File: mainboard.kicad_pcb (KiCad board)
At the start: 2 copper layers, 115.3 x 64.5 mm, 13 parts

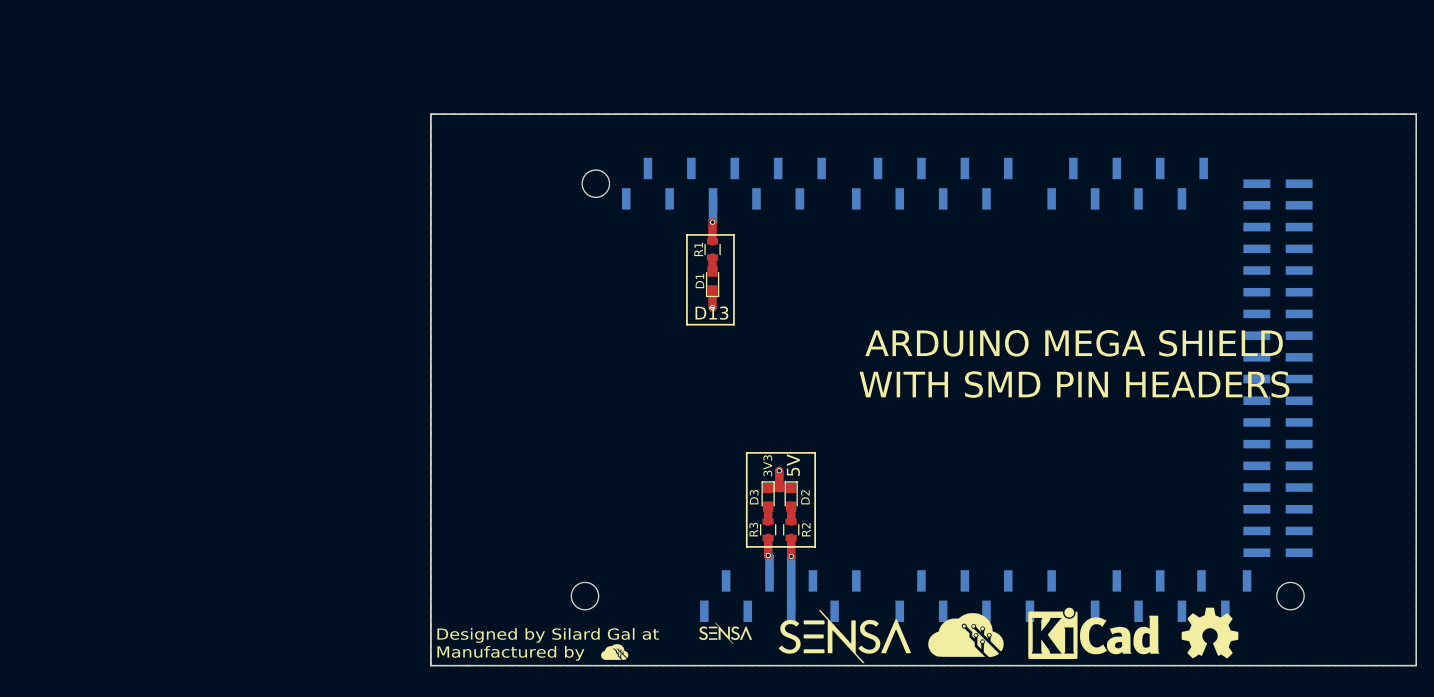
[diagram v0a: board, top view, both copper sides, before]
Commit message: Beta version
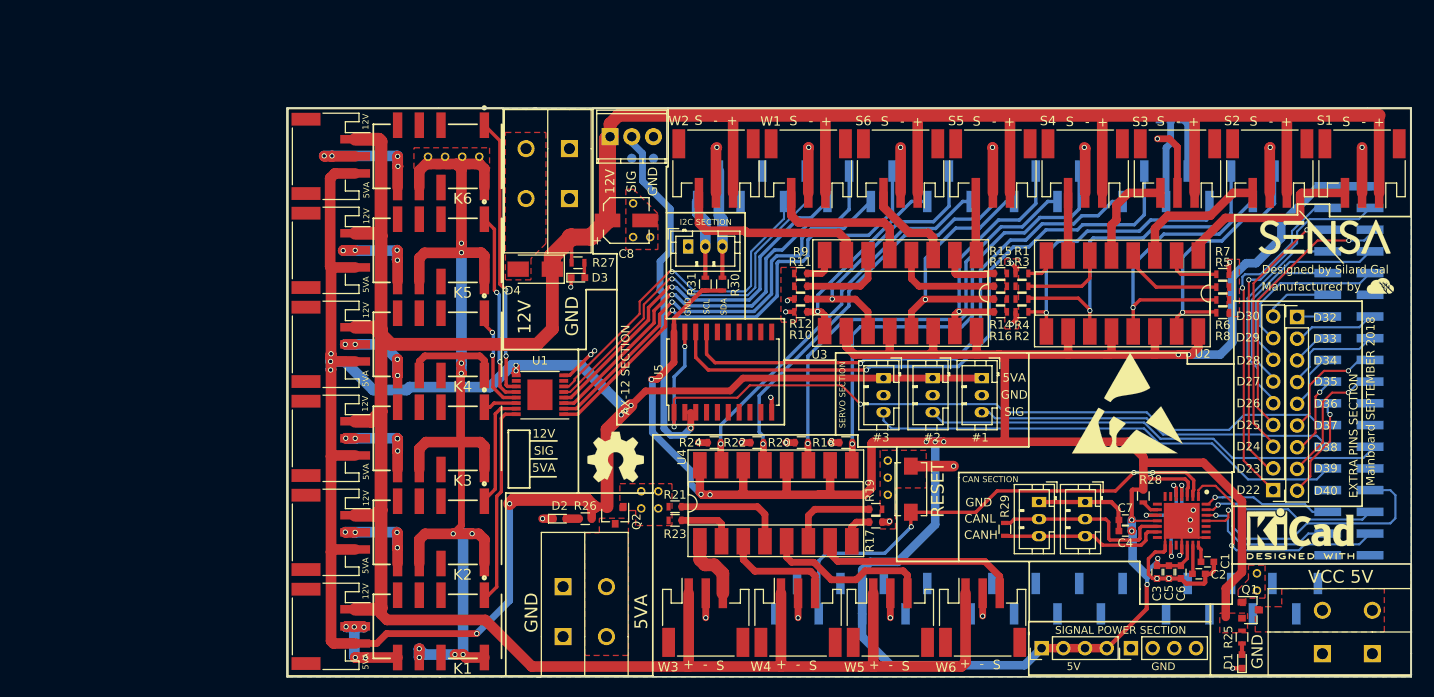
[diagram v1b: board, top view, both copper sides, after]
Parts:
- removed the G*** at (219.8, 140.8)
- removed the G*** at (191.4, 140.6)
- removed the REF*** at (234.6, 140.6)
- added C1: C, Capacitors_SMD:C_0603, F.Cu at (247.9, 132.2)
- added C2: C, Capacitors_SMD:C_0603, F.Cu at (246.9, 133.7)
- added C3: 10u, Capacitors_SMD:C_0603, F.Cu at (242.0, 133.4)
- added C4: 0.1u, Capacitors_SMD:C_0603, F.Cu at (238.3, 128.7)
- added C5: 0.1u, Capacitors_SMD:C_0603, F.Cu at (243.4, 133.4)
- added C6: 0.1u, Capacitors_SMD:C_0603, F.Cu at (244.8, 133.4)
- added C7: 0.1u, Capacitors_SMD:C_0603, F.Cu at (238.3, 127.3)
- added C8: CP, Capacitors_SMD:CP_Elec_5x5.8, F.Cu at (179.9, 92.3)
- added D4: D, Diodes_SMD:D_SMA, F.Cu at (169.2, 98.0)
- added IC1: MCP25625-E_ML, MCP25625-E_ML:QFN65P600X600X100-29N-D, F.Cu at (244.9, 127.5)
- added J1: SENS1, Connectors_JST:JST_PH_S3B-PH-SM4-TB_03x2.00mm_Angled, F.Cu at (266.0, 86.2)
- added J10: R4, Connectors_JST:JST_PH_S3B-PH-SM4-TB_03x2.00mm_Angled, F.Cu at (145.3, 106.8)
- added J11: R5, Connectors_JST:JST_PH_S3B-PH-SM4-TB_03x2.00mm_Angled, F.Cu at (145.3, 95.8)
- added J12: R6, Connectors_JST:JST_PH_S3B-PH-SM4-TB_03x2.00mm_Angled, F.Cu at (145.3, 84.8)
- added J13: SW1, Connectors_JST:JST_PH_S3B-PH-SM4-TB_03x2.00mm_Angled, F.Cu at (201.2, 86.2)
- added J14: SW2, Connectors_JST:JST_PH_S3B-PH-SM4-TB_03x2.00mm_Angled, F.Cu at (190.4, 86.2)
- added J15: SW3, Connectors_JST:JST_PH_S3B-PH-SM4-TB_03x2.00mm_Angled, F.Cu at (189.2, 138.8)
- added J16: SW4, Connectors_JST:JST_PH_S3B-PH-SM4-TB_03x2.00mm_Angled, F.Cu at (200.0, 138.8)
- added J17: SW5, Connectors_JST:JST_PH_S3B-PH-SM4-TB_03x2.00mm_Angled, F.Cu at (210.8, 138.8)
- added J18: SW6, Connectors_JST:JST_PH_S3B-PH-SM4-TB_03x2.00mm_Angled, F.Cu at (221.6, 138.8)
- added J19: Conn_01x03, Connectors_JST:JST_PH_B3B-PH-K_03x2.00mm_Straight, F.Cu at (221.5, 110.8)
- added J2: SENS2, Connectors_JST:JST_PH_S3B-PH-SM4-TB_03x2.00mm_Angled, F.Cu at (255.2, 86.2)
- added J20: Conn_01x03, Connectors_JST:JST_PH_B3B-PH-K_03x2.00mm_Straight, F.Cu at (215.8, 110.8)
- added J21: Conn_01x03, Connectors_JST:JST_PH_B3B-PH-K_03x2.00mm_Straight, F.Cu at (210.0, 110.8)
- added J22: Conn_01x03, Connectors_JST:JST_PH_B3B-PH-K_03x2.00mm_Straight, F.Cu at (187.2, 95.3)
- added J23: Screw_Terminal_01x02, Custom Connector:ZFKDS, F.Cu at (267.2, 143.0)
- added J24: Screw_Terminal_01x02, Custom Connector:ZFKDS, F.Cu at (172.5, 141.0)
- added J25: Screw_Terminal_01x02, Custom Connector:ZFKDS, F.Cu at (173.2, 83.9)
- added J26: Conn_01x03, Connectors_JST:JST_PH_B3B-PH-K_03x2.00mm_Straight, F.Cu at (233.6, 125.2)
- added J27: Conn_01x03, Connectors_JST:JST_PH_B3B-PH-K_03x2.00mm_Straight, F.Cu at (228.2, 125.2)
- added J28: Conn_01x04, Pin_Headers:Pin_Header_Straight_1x04_Pitch2.54mm, F.Cu at (228.5, 142.3)
- added J29: Conn_01x03, Connectors:GS3, B.Cu at (243.6, 80.3)
- added J3: SENS3, Connectors_JST:JST_PH_S3B-PH-SM4-TB_03x2.00mm_Angled, F.Cu at (244.4, 86.2)
- added J30: Screw_Terminal_01x03, TerminalBlocks_Phoenix:TerminalBlock_Phoenix_MPT-2.54mm_3pol, F.Cu at (178.0, 82.5)
- added J31: Conn_01x04, Pin_Headers:Pin_Header_Straight_1x04_Pitch2.54mm, F.Cu at (238.9, 142.3)
- added J32: Conn_01x10, Pin_Headers:Pin_Header_Straight_1x09_Pitch2.54mm, F.Cu at (255.6, 123.8)
- added J33: Conn_01x10, Pin_Headers:Pin_Header_Straight_1x09_Pitch2.54mm, F.Cu at (258.4, 103.6)
- added J4: SENS4, Connectors_JST:JST_PH_S3B-PH-SM4-TB_03x2.00mm_Angled, F.Cu at (233.6, 86.2)
- added J5: SENS5, Connectors_JST:JST_PH_S3B-PH-SM4-TB_03x2.00mm_Angled, F.Cu at (222.8, 86.2)
- added J6: SENS6, Connectors_JST:JST_PH_S3B-PH-SM4-TB_03x2.00mm_Angled, F.Cu at (212.0, 86.2)
- added J7: R1, Connectors_JST:JST_PH_S3B-PH-SM4-TB_03x2.00mm_Angled, F.Cu at (145.3, 139.8)
- added J8: R2, Connectors_JST:JST_PH_S3B-PH-SM4-TB_03x2.00mm_Angled, F.Cu at (145.3, 128.8)
- added J9: R3, Connectors_JST:JST_PH_S3B-PH-SM4-TB_03x2.00mm_Angled, F.Cu at (145.3, 117.8)
- added K1: EE2-5NU, EE2-5NU, F.Cu at (165.3, 139.8)
- added K2: EE2-5NU, EE2-5NU, F.Cu at (165.3, 128.8)
- added K3: EE2-5NU, EE2-5NU, F.Cu at (165.3, 117.8)
- added K4: EE2-5NU, EE2-5NU, F.Cu at (165.3, 106.8)
- added K5: EE2-5NU, EE2-5NU, F.Cu at (165.3, 95.8)
- added K6: EE2-5NU, EE2-5NU, F.Cu at (165.3, 84.8)
- added Q1: DMP2100U, TO_SOT_Packages_SMD:SOT-23, F.Cu at (252.9, 137.9)
- added Q2: DMP2100U, TO_SOT_Packages_SMD:SOT-23, F.Cu at (178.6, 126.8)
- added R10: 4k7, Resistors_SMD:R_0603, F.Cu at (200.3, 103.0)
- added R11: 330, Resistors_SMD:R_0603, F.Cu at (200.3, 100.0)
- added R12: 4k7, Resistors_SMD:R_0603, F.Cu at (200.3, 101.5)
- added R13: 330, Resistors_SMD:R_0603, F.Cu at (223.7, 100.0)
- added R14: 4k7, Resistors_SMD:R_0603, F.Cu at (223.7, 101.5)
- added R15: 330, Resistors_SMD:R_0603, F.Cu at (223.7, 98.5)
- added R16: 4k7, Resistors_SMD:R_0603, F.Cu at (223.7, 103.0)
- added R17: 330, Resistors_SMD:R_0603, F.Cu at (209.1, 127.6)
- added R18: 4k7, Resistors_SMD:R_0603, F.Cu at (205.6, 118.3)
- added R19: 330, Resistors_SMD:R_0603, F.Cu at (209.1, 126.1)
- added R20: 4k7, Resistors_SMD:R_0603, F.Cu at (200.4, 118.3)
- added R21: 330, Resistors_SMD:R_0603, F.Cu at (185.6, 125.8)
- added R22: 4k7, Resistors_SMD:R_0603, F.Cu at (195.2, 118.3)
- added R23: 330, Resistors_SMD:R_0603, F.Cu at (185.6, 127.4)
- added R24: 4k7, Resistors_SMD:R_0603, F.Cu at (190.2, 118.3)
- added R25: 330, Resistors_SMD:R_0603, F.Cu at (251.9, 141.1)
- added R26: 330, Resistors_SMD:R_0603, F.Cu at (175.1, 127.2)
- added R27: 1K, Resistors_SMD:R_0603, F.Cu at (174.2, 97.2)
- added R28: 10k, Resistors_SMD:R_0603, F.Cu at (240.4, 124.5)
- added R29: 120, Resistors_SMD:R_0603, F.Cu at (224.2, 128.4)
- added R30: 4k7, Resistors_SMD:R_0603, F.Cu at (191.2, 99.8)
- added R31: 4k7, Resistors_SMD:R_0603, F.Cu at (189.2, 99.8)
- added R4: 4k7, Resistors_SMD:R_0603, F.Cu at (226.2, 101.5)
- added R5: 330, Resistors_SMD:R_0603, F.Cu at (249.7, 100.1)
- added R6: 4k7, Resistors_SMD:R_0603, F.Cu at (249.7, 101.6)
- added R7: 330, Resistors_SMD:R_0603, F.Cu at (249.7, 98.6)
- added R8: 4k7, Resistors_SMD:R_0603, F.Cu at (249.7, 103.1)
- added R9: 330, Resistors_SMD:R_0603, F.Cu at (200.3, 98.5)
- added REF**: SolderWirePad_single_1mmDrill, Wire_Pads:SolderWirePad_single_1mmDrill, F.Cu at (182.7, 94.2)
- added REF**: SolderWirePad_single_1mmDrill, Wire_Pads:SolderWirePad_single_1mmDrill, F.Cu at (253.7, 135.6)
- added REF**: SolderWirePad_single_1mmDrill, Wire_Pads:SolderWirePad_single_1mmDrill, F.Cu at (183.7, 126.0)
- added REF**: SolderWirePad_single_1mmDrill, Wire_Pads:SolderWirePad_single_1mmDrill, F.Cu at (181.7, 126.0)
- added REF**: SolderWirePad_single_1mmDrill, Wire_Pads:SolderWirePad_single_1mmDrill, F.Cu at (210.5, 120.4)
- added REF**: SolderWirePad_single_1mmDrill, Wire_Pads:SolderWirePad_single_1mmDrill, F.Cu at (253.7, 133.6)
- added REF**: SolderWirePad_single_1mmDrill, Wire_Pads:SolderWirePad_single_1mmDrill, F.Cu at (183.7, 124.0)
- added REF**: SolderWirePad_single_1mmDrill, Wire_Pads:SolderWirePad_single_1mmDrill, F.Cu at (181.7, 124.0)
- added REF**: SolderWirePad_single_1mmDrill, Wire_Pads:SolderWirePad_single_1mmDrill, F.Cu at (180.7, 94.2)
- added REF**: SolderWirePad_single_1mmDrill, Wire_Pads:SolderWirePad_single_1mmDrill, F.Cu at (180.7, 90.3)
- added REF**: SolderWirePad_single_1mmDrill, Wire_Pads:SolderWirePad_single_1mmDrill, F.Cu at (162.7, 84.8)
- added REF**: SolderWirePad_single_1mmDrill, Wire_Pads:SolderWirePad_single_1mmDrill, F.Cu at (160.7, 84.8)
- added REF**: SolderWirePad_single_1mmDrill, Wire_Pads:SolderWirePad_single_1mmDrill, F.Cu at (158.7, 84.8)
- added REF**: SolderWirePad_single_1mmDrill, Wire_Pads:SolderWirePad_single_1mmDrill, F.Cu at (156.7, 84.8)
- added REF**: SolderWirePad_single_1mmDrill, Wire_Pads:SolderWirePad_single_1mmDrill, F.Cu at (210.5, 124.4)
- added REF**: SolderWirePad_single_1mmDrill, Wire_Pads:SolderWirePad_single_1mmDrill, F.Cu at (210.5, 122.4)
- added REF***: ESD-Logo_13.2x12mm_SilkScreen, Symbols:ESD-Logo_13.2x12mm_SilkScreen, F.Cu at (238.6, 113.7)
- added REF***: KiCad-Logo2_6mm_SilkScreen, Symbols:KiCad-Logo2_6mm_SilkScreen, F.Cu at (258.8, 128.9)
- added SW1: SW_Push, Buttons_Switches_SMD:SW_SPST_EVQPE1, F.Cu at (213.2, 123.8)
- added U1: ULN2003A, Housings_SSOP:TSSOP-16-1EP_4.4x5mm_Pitch0.65mm, F.Cu at (169.8, 112.7)
- added U2: LTV-847, Housings_DIP:DIP-16_W8.89mm_SMDSocket_LongPads, F.Cu at (237.9, 100.8)
- added U3: LTV-847, Housings_DIP:DIP-16_W8.89mm_SMDSocket_LongPads, F.Cu at (212.0, 100.8)
- added U4: LTV-847, Housings_DIP:DIP-16_W8.89mm_SMDSocket_LongPads, F.Cu at (197.4, 125.4)
- added U5: 74LS241, Housings_SOIC:SOIC-20W_7.5x12.8mm_Pitch1.27mm, F.Cu at (191.2, 110.0)
- D1, D2, D3: footprint LEDs:LED_0805 -> LEDs:LED_0603
- R1, R3: value R -> 330; footprint Resistors_SMD:R_0805 -> Resistors_SMD:R_0603
- R2: value R -> 4k7; footprint Resistors_SMD:R_0805 -> Resistors_SMD:R_0603
- moved G*** 99.3 mm to (268.2, 100.0)
- moved D1 76.3 mm to (251.9, 143.9)
- moved G*** 73.1 mm to (261.4, 94.2)
- moved REF*** 72.5 mm to (178.7, 120.0)
- moved R3 41.2 mm to (226.2, 100.0), turned to 0 degrees
- moved R2 37.1 mm to (226.2, 103.0), turned to 180 degrees
- moved R1 36.3 mm to (226.2, 98.5), turned to 0 degrees
- moved D3 34.0 mm to (174.2, 99.0), turned to 0 degrees
- moved D2 27.2 mm to (172.1, 127.2), turned to 0 degrees
- moved XA1 8.31 mm to (169.4, 139.1)
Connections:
- R1 pad 1: D13 -> GND
- R1 pad 2: Net-(D1-Pad2) -> Net-(R1-Pad2)
- R2 pad 1: +5V -> SO_4
- R2 pad 2: Net-(D2-Pad2) -> GND
- R3 pad 1: +3V3 -> GND
- R3 pad 2: Net-(D3-Pad2) -> Net-(R3-Pad2)
- XA1 pad 3V3: +3V3 -> (no net)
- XA1 pad D0: (no net) -> SWO_6
- XA1 pad D1: (no net) -> SWO_5
- XA1 pad D10: (no net) -> R3_CONT
- XA1 pad D11: (no net) -> R4_CONT
- XA1 pad D12: (no net) -> R5_CONT
- XA1 pad D13: D13 -> R6_CONT
- XA1 pad D14: (no net) -> AX_TX
- XA1 pad D15: (no net) -> AX_RX
- XA1 pad D16: (no net) -> DBG_TX
- XA1 pad D17: (no net) -> DBG_RX
- XA1 pad D18: (no net) -> SO_4
- XA1 pad D19: (no net) -> SO_3
- XA1 pad D2: (no net) -> SO_5
- XA1 pad D20: (no net) -> SO_2
- XA1 pad D21: (no net) -> SO_1
- XA1 pad D22: (no net) -> Net-(J32-Pad1)
- XA1 pad D23: (no net) -> Net-(J32-Pad2)
- XA1 pad D24: (no net) -> Net-(J32-Pad3)
- XA1 pad D25: (no net) -> Net-(J32-Pad4)
- XA1 pad D26: (no net) -> Net-(J32-Pad5)
- XA1 pad D27: (no net) -> Net-(J32-Pad6)
- XA1 pad D28: (no net) -> Net-(J32-Pad7)
- XA1 pad D29: (no net) -> Net-(J32-Pad8)
- XA1 pad D3: (no net) -> SO_6
- XA1 pad D30: (no net) -> Net-(J32-Pad9)
- XA1 pad D32: (no net) -> Net-(J33-Pad1)
- XA1 pad D33: (no net) -> Net-(J33-Pad2)
- XA1 pad D34: (no net) -> Net-(J33-Pad3)
- XA1 pad D35: (no net) -> Net-(J33-Pad4)
- XA1 pad D36: (no net) -> Net-(J33-Pad5)
- XA1 pad D37: (no net) -> Net-(J33-Pad6)
- XA1 pad D38: (no net) -> Net-(J33-Pad7)
- XA1 pad D39: (no net) -> Net-(J33-Pad8)
- XA1 pad D4: (no net) -> SWO_4
- XA1 pad D40: (no net) -> Net-(J33-Pad9)
- XA1 pad D42: (no net) -> AX_CONTROL
- XA1 pad D44: (no net) -> PWM1
- XA1 pad D45: (no net) -> PWM2
- XA1 pad D46: (no net) -> PWM3
- XA1 pad D49: (no net) -> CAN_INT
- XA1 pad D5: (no net) -> SWO_3
- XA1 pad D50: (no net) -> CAN_MISO
- XA1 pad D51: (no net) -> CAN_MOSI
- XA1 pad D52: (no net) -> CAN_SCK
- XA1 pad D53: (no net) -> CAN_CS
- XA1 pad D6: (no net) -> SWO_1
- XA1 pad D7: (no net) -> SWO_2
- XA1 pad D8: (no net) -> R1_CONT
- XA1 pad D9: (no net) -> R2_CONT
- XA1 pad GND1: (no net) -> GND
- XA1 pad GND2: (no net) -> GND
- XA1 pad GND3: (no net) -> GND
- XA1 pad GND5: (no net) -> GND
- XA1 pad GND6: (no net) -> GND
- XA1 pad RST1: (no net) -> RST
- XA1 pad SCL: (no net) -> SCL
- XA1 pad SDA: (no net) -> SDA
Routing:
- net +12V: track 0.00 -> 404.7 mm
- net +5V: track 8.59 -> 353.5 mm, vias 1 -> 12
- net +5VA: track 0.00 -> 269.2 mm, vias 0 -> 10
- net GND: track 6.70 -> 274.9 mm, vias 2 -> 45
- net AX_CONTROL: track 0.00 -> 95.4 mm, vias 0 -> 3
- net AX_RX: track 0.00 -> 73.1 mm, vias 0 -> 1
- net AX_TX: track 0.00 -> 64.0 mm, vias 0 -> 1
- net RST: track 0.00 -> 57.7 mm, vias 0 -> 3
- net R1_CONT: track 0.00 -> 57.7 mm, vias 0 -> 1
- net PWM3: track 0.00 -> 56.3 mm
- net SWO_6: track 0.00 -> 56.2 mm, vias 0 -> 1
- net PWM2: track 0.00 -> 55.7 mm
- net SWO_5: track 0.00 -> 53.3 mm, vias 0 -> 1
- net R3_CONT: track 0.00 -> 51.5 mm, vias 0 -> 1
- net R2_CONT: track 0.00 -> 50.9 mm, vias 0 -> 1
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- added copper zone on F.Cu, net +5V
- added copper zone on F.Cu, net GND
- added copper zone on F.Cu, net Net-(D4-Pad2)
- added copper zone on F.Cu, net Net-(J23-Pad2)
- added copper zone on F.Cu, net Net-(J24-Pad2)
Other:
- board size 115.3 x 64.5 mm -> 131.6 x 66.5 mm
- board text added: "#1"
- board text added: "#2"
- board text added: "#3"
- board text added: "+"
- board text added: "-"
- board text added: "12V"
- board text added: "5VA"
- board text added: "AX-12 SECTION"
- board text added: "CAN SECTION"
- board text added: "CANH"
- board text added: "CANL"
- board text added: "D22"
- board text added: "D23"
- board text added: "D24"
- board text added: "D25"
- board text added: "D26"
- board text added: "D27"
- board text added: "D28"
- board text added: "D29"
- board text added: "D30"
- board text added: "D32"
- board text added: "D33"
- board text added: "D34"
- board text added: "D35"
- board text added: "D36"
- board text added: "D37"
- board text added: "D38"
- board text added: "D39"
- board text added: "D40"
- board text added: "Designed by Silard Gal"
- board text added: "EXTRA PINS SECTION"
- board text added: "GND"
- board text added: "I2C SECTION"
- board text added: "Mainboard SEPTEMBER 2018"
- board text added: "Manufactured by"
- board text added: "RESET"
- board text added: "S"
- board text added: "S1"
- board text added: "S2"
- board text added: "S3"
- board text added: "S4"
- board text added: "S5"
- board text added: "S6"
- board text added: "SCL"
- board text added: "SDA"
- board text added: "SERVO SECTION"
- board text added: "SIG"
- board text added: "SIGNAL POWER SECTION"
- board text added: "VCC 5V"
- board text added: "W1"
- board text added: "W2"
- board text added: "W3"
- board text added: "W4"
- board text added: "W5"
- board text added: "W6"
- board text removed: "3V3"
- board text removed: "ARDUINO MEGA SHIELD WITH SMD PIN HEADERS"
- board text removed: "D13"
- board text removed: "Designed by Silard Gal at Manufactured by"

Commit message: Finished version 1.0
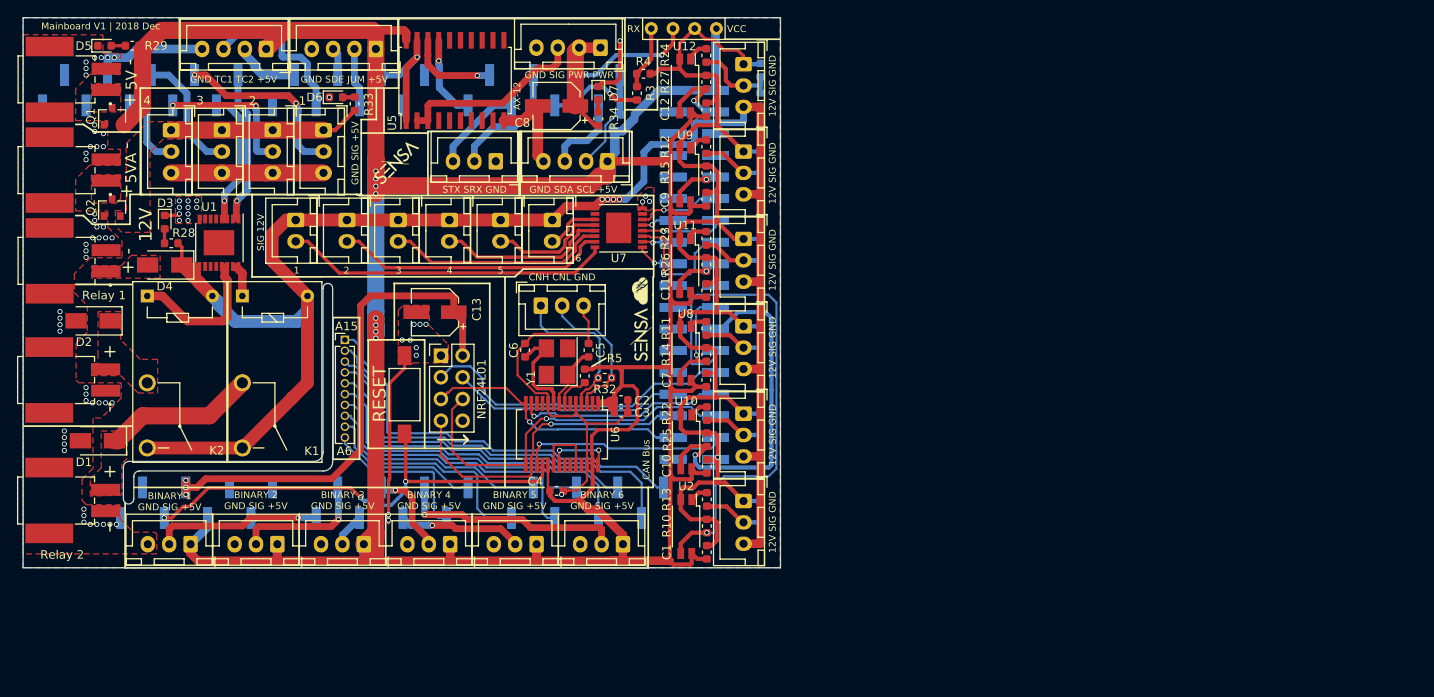
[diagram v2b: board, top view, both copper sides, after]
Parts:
- removed IC1: MCP25625-E_ML, MCP25625-E_ML:QFN65P600X600X100-29N-D
- removed J16: SW4, Connectors_JST:JST_PH_S3B-PH-SM4-TB_03x2.00mm_Angled
- removed J29: Conn_01x03, Connectors:GS3
- removed K3, K4, K5, K6: EE2-5NU, EE2-5NU
- removed REF** (x16): SolderWirePad_single_1mmDrill, Wire_Pads:SolderWirePad_single_1mmDrill
- removed REF***: ESD-Logo_13.2x12mm_SilkScreen, Symbols:ESD-Logo_13.2x12mm_SilkScreen
- removed REF***: KiCad-Logo2_6mm_SilkScreen, Symbols:KiCad-Logo2_6mm_SilkScreen
- removed REF***: OSHW-Symbol_6.7x6mm_SilkScreen, Symbols:OSHW-Symbol_6.7x6mm_SilkScreen
- removed SW1: SW_Push, Buttons_Switches_SMD:SW_SPST_EVQPE1
- removed the XA1 at (169.4, 139.1)
- added C10: 100n, Capacitor_SMD:C_0603_1608Metric, F.Cu at (189.3, 121.1)
- added C11: 100n, Capacitor_SMD:C_0603_1608Metric, F.Cu at (189.3, 100.5)
- added C12: 100n, Capacitor_SMD:C_0603_1608Metric, F.Cu at (189.3, 79.3)
- added C13: CP, Capacitor_SMD:CP_Elec_5x5.8, F.Cu at (157.5, 103.0)
- added C9: 100n, Capacitor_SMD:C_0603_1608Metric, F.Cu at (189.3, 89.8)
- added D5: LED, LED_SMD:LED_0603_1608Metric, F.Cu at (118.8, 71.9)
- added D6: LED, LED_SMD:LED_0603_1608Metric, F.Cu at (145.9, 77.9)
- added D7: LED, LED_SMD:LED_0603_1608Metric, F.Cu at (176.6, 77.4)
- added G***: LOGO, logos:SENSA_6x3, F.Cu at (152.9, 85.5)
- added G***: LOGO, logos:SENSA_6x3, F.Cu at (181.6, 105.8)
- added G***: LOGO, logos:AISLER_9x5, B.Cu at (173.0, 119.0)
- added J34: SERVO4, Connector_JST:JST_XH_B03B-XH-A_1x03_P2.50mm_Vertical, F.Cu at (126.6, 81.7)
- added J35: RELAY2, PHOENIX_1702473, F.Cu at (113.2, 111.0)
- added J36: RELAY1, PHOENIX_1702473, F.Cu at (113.2, 125.1)
- added R32: 120, Resistor_SMD:R_0603_1608Metric, F.Cu at (177.4, 110.7)
- added R33: 1K, Resistor_SMD:R_0603_1608Metric, F.Cu at (148.1, 78.7)
- added R34: 1K, Resistor_SMD:R_0603_1608Metric, F.Cu at (176.6, 80.4)
- added RESET1: SW_Push, Button_Switch_SMD:SW_SPST_FSMSM, F.Cu at (154.0, 112.7)
- added U10: PC817, Package_SO:SOP-4_4.4x2.8mm_P1.27mm, F.Cu at (186.9, 118.2)
- added U11: PC817, Package_SO:SOP-4_4.4x2.8mm_P1.27mm, F.Cu at (186.8, 97.6)
- added U12: PC817, Package_SO:SOP-4_4.4x2.8mm_P1.27mm, F.Cu at (186.8, 76.6)
- added U6: MCP25625-x-SS, Package_SO:SSOP-28_5.3x10.2mm_P0.65mm, F.Cu at (172.4, 117.3)
- added U7: ULN2003A, Package_SO:TSSOP-16-1EP_4.4x5mm_P0.65mm, F.Cu at (179.0, 93.2)
- added U8: PC817, Package_SO:SOP-4_4.4x2.8mm_P1.27mm, F.Cu at (186.9, 107.9)
- added U9: PC817, Package_SO:SOP-4_4.4x2.8mm_P1.27mm, F.Cu at (186.8, 87.0)
- added XA1 (x2): Arduino_Mega2560_Shield, Arduino:Arduino_Mega2560_Shield, F.Cu at (92.8, 127.9)
- added Y1: Crystal_GND24, Crystal:Crystal_SMD_SeikoEpson_FA238V-4Pin_3.2x2.5mm_HandSoldering, F.Cu at (171.8, 108.8)
- C1: value C -> 100n; footprint Capacitors_SMD:C_0603 -> Capacitor_SMD:C_0603_1608Metric
- C2: value C -> 10u; footprint Capacitors_SMD:C_0603 -> Capacitor_SMD:C_0603_1608Metric
- C3: value 10u -> 100n; footprint Capacitors_SMD:C_0603 -> Capacitor_SMD:C_0603_1608Metric
- C4: value 0.1u -> 10u; footprint Capacitors_SMD:C_0603 -> Capacitor_SMD:C_0603_1608Metric
- C5, C6: value 0.1u -> 20p; footprint Capacitors_SMD:C_0603 -> Capacitor_SMD:C_0603_1608Metric
- C7: value 0.1u -> 100n; footprint Capacitors_SMD:C_0603 -> Capacitor_SMD:C_0603_1608Metric
- C8: footprint Capacitors_SMD:CP_Elec_5x5.8 -> Capacitor_SMD:CP_Elec_5x5.8
- D1, D2: value LED -> D; footprint LEDs:LED_0603 -> Diode_SMD:D_SMA
- D3: footprint LEDs:LED_0603 -> LED_SMD:LED_0603_1608Metric
- D4: footprint Diodes_SMD:D_SMA -> Diode_SMD:D_SMA
- G***: moved to B.Cu
- J1: value SENS1 -> Conn_01x10; footprint Connectors_JST:JST_PH_S3B-PH-SM4-TB_03x2.00mm_Angled -> Connector_PinHeader_1.27mm:PinHeader_1x10_P1.27mm_Vertical
- J10: value R4 -> jump_side; footprint Connectors_JST:JST_PH_S3B-PH-SM4-TB_03x2.00mm_Angled -> Connector_JST:JST_XH_B04B-XH-A_1x04_P2.50mm_Vertical
- J11: value R5 -> Senzor1; footprint Connectors_JST:JST_PH_S3B-PH-SM4-TB_03x2.00mm_Angled -> Connector_JST:JST_XH_B03B-XH-A_1x03_P2.50mm_Vertical
- J12: value R6 -> tactics_sw; footprint Connectors_JST:JST_PH_S3B-PH-SM4-TB_03x2.00mm_Angled -> Connector_JST:JST_XH_B04B-XH-A_1x04_P2.50mm_Vertical
- J13: value SW1 -> i2c_con; footprint Connectors_JST:JST_PH_S3B-PH-SM4-TB_03x2.00mm_Angled -> Connector_JST:JST_XH_B04B-XH-A_1x04_P2.50mm_Vertical
- J14: value SW2 -> ser_con; footprint Connectors_JST:JST_PH_S3B-PH-SM4-TB_03x2.00mm_Angled -> Connector_JST:JST_XH_B03B-XH-A_1x03_P2.50mm_Vertical
- J15: value SW3 -> CAN; footprint Connectors_JST:JST_PH_S3B-PH-SM4-TB_03x2.00mm_Angled -> Connector_JST:JST_XH_B03B-XH-A_1x03_P2.50mm_Vertical
- J17: value SW5 -> Senzor3; footprint Connectors_JST:JST_PH_S3B-PH-SM4-TB_03x2.00mm_Angled -> Connector_JST:JST_XH_B03B-XH-A_1x03_P2.50mm_Vertical
- J18: value SW6 -> Senzor5; footprint Connectors_JST:JST_PH_S3B-PH-SM4-TB_03x2.00mm_Angled -> Connector_JST:JST_XH_B03B-XH-A_1x03_P2.50mm_Vertical
- J19: value Conn_01x03 -> SERVO1; footprint Connectors_JST:JST_PH_B3B-PH-K_03x2.00mm_Straight -> Connector_JST:JST_XH_B03B-XH-A_1x03_P2.50mm_Vertical
- J2: value SENS2 -> AX; footprint Connectors_JST:JST_PH_S3B-PH-SM4-TB_03x2.00mm_Angled -> Connector_JST:JST_XH_B04B-XH-A_1x04_P2.50mm_Vertical
- J20: value Conn_01x03 -> SERVO2; footprint Connectors_JST:JST_PH_B3B-PH-K_03x2.00mm_Straight -> Connector_JST:JST_XH_B03B-XH-A_1x03_P2.50mm_Vertical
- J21: value Conn_01x03 -> S2; footprint Connectors_JST:JST_PH_B3B-PH-K_03x2.00mm_Straight -> Connector_JST:JST_XH_B02B-XH-A_1x02_P2.50mm_Vertical
- J22: value Conn_01x03 -> S3; footprint Connectors_JST:JST_PH_B3B-PH-K_03x2.00mm_Straight -> Connector_JST:JST_XH_B02B-XH-A_1x02_P2.50mm_Vertical
- J23: value Screw_Terminal_01x02 -> 12V_IN; footprint Custom Connector:ZFKDS -> PHOENIX_1702473
- J24: value Screw_Terminal_01x02 -> 5V_IN; footprint Custom Connector:ZFKDS -> PHOENIX_1702473
- J25: value Screw_Terminal_01x02 -> 5VA_IN; footprint Custom Connector:ZFKDS -> PHOENIX_1702473
- J26: value Conn_01x03 -> S4; footprint Connectors_JST:JST_PH_B3B-PH-K_03x2.00mm_Straight -> Connector_JST:JST_XH_B02B-XH-A_1x02_P2.50mm_Vertical
- J27: value Conn_01x03 -> S5; footprint Connectors_JST:JST_PH_B3B-PH-K_03x2.00mm_Straight -> Connector_JST:JST_XH_B02B-XH-A_1x02_P2.50mm_Vertical
- J28: value Conn_01x04 -> S6; footprint Pin_Headers:Pin_Header_Straight_1x04_Pitch2.54mm -> Connector_JST:JST_XH_B02B-XH-A_1x02_P2.50mm_Vertical
- J3: value SENS3 -> bin_sens1; footprint Connectors_JST:JST_PH_S3B-PH-SM4-TB_03x2.00mm_Angled -> Connector_JST:JST_XH_B03B-XH-A_1x03_P2.50mm_Vertical
- J30: value Screw_Terminal_01x03 -> Senzor2; footprint TerminalBlocks_Phoenix:TerminalBlock_Phoenix_MPT-2.54mm_3pol -> Connector_JST:JST_XH_B03B-XH-A_1x03_P2.50mm_Vertical
- J31: value Conn_01x04 -> Senzor4; footprint Pin_Headers:Pin_Header_Straight_1x04_Pitch2.54mm -> Connector_JST:JST_XH_B03B-XH-A_1x03_P2.50mm_Vertical
- J32: value Conn_01x10 -> Senzor6; footprint Pin_Headers:Pin_Header_Straight_1x09_Pitch2.54mm -> Connector_JST:JST_XH_B03B-XH-A_1x03_P2.50mm_Vertical
- J33: value Conn_01x10 -> SERVO3; footprint Pin_Headers:Pin_Header_Straight_1x09_Pitch2.54mm -> Connector_JST:JST_XH_B03B-XH-A_1x03_P2.50mm_Vertical
- J4: value SENS4 -> bin_sens4; footprint Connectors_JST:JST_PH_S3B-PH-SM4-TB_03x2.00mm_Angled -> Connector_JST:JST_XH_B03B-XH-A_1x03_P2.50mm_Vertical
- J5: value SENS5 -> S1; footprint Connectors_JST:JST_PH_S3B-PH-SM4-TB_03x2.00mm_Angled -> Connector_JST:JST_XH_B02B-XH-A_1x02_P2.50mm_Vertical
- J6: value SENS6 -> bin_sens2; footprint Connectors_JST:JST_PH_S3B-PH-SM4-TB_03x2.00mm_Angled -> Connector_JST:JST_XH_B03B-XH-A_1x03_P2.50mm_Vertical
- J7: value R1 -> bin_sens5; footprint Connectors_JST:JST_PH_S3B-PH-SM4-TB_03x2.00mm_Angled -> Connector_JST:JST_XH_B03B-XH-A_1x03_P2.50mm_Vertical
- J8: value R2 -> bin_sens3; footprint Connectors_JST:JST_PH_S3B-PH-SM4-TB_03x2.00mm_Angled -> Connector_JST:JST_XH_B03B-XH-A_1x03_P2.50mm_Vertical
- J9: value R3 -> bin_sens6; footprint Connectors_JST:JST_PH_S3B-PH-SM4-TB_03x2.00mm_Angled -> Connector_JST:JST_XH_B03B-XH-A_1x03_P2.50mm_Vertical
- K1, K2: value EE2-5NU -> G5Q-1A; footprint EE2-5NU -> Relay_THT:Relay_SPST_Omron-G5Q-1A
- Q1, Q2: footprint TO_SOT_Packages_SMD:SOT-23 -> Package_TO_SOT_SMD:SOT-23
- R1: value 330 -> 500; footprint Resistors_SMD:R_0603 -> Resistor_SMD:R_0603_1608Metric; moved to B.Cu
- R10, R14: value 4k7 -> 10K; footprint Resistors_SMD:R_0603 -> Resistor_SMD:R_0603_1608Metric
- R11, R13, R23: value 330 -> 500; footprint Resistors_SMD:R_0603 -> Resistor_SMD:R_0603_1608Metric
- R12, R22, R24: value 4k7 -> 500; footprint Resistors_SMD:R_0603 -> Resistor_SMD:R_0603_1608Metric
- R15, R25, R26, R5: value 330 -> 10K; footprint Resistors_SMD:R_0603 -> Resistor_SMD:R_0603_1608Metric
- R16, R18, R20, R6, R8: value 4k7 -> 500; footprint Resistors_SMD:R_0603 -> Resistor_SMD:R_0603_1608Metric; moved to B.Cu
- R17, R19, R21, R7, R9: value 330 -> 1K; footprint Resistors_SMD:R_0603 -> Resistor_SMD:R_0603_1608Metric; moved to B.Cu
- R2: value 4k7 -> 1K; footprint Resistors_SMD:R_0603 -> Resistor_SMD:R_0603_1608Metric; moved to B.Cu
- R27: value 1K -> 10K; footprint Resistors_SMD:R_0603 -> Resistor_SMD:R_0603_1608Metric
- R28: value 10k -> 1K; footprint Resistors_SMD:R_0603 -> Resistor_SMD:R_0603_1608Metric
- R29: value 120 -> 1K; footprint Resistors_SMD:R_0603 -> Resistor_SMD:R_0603_1608Metric
- R3: value 330 -> 1K; footprint Resistors_SMD:R_0603 -> Resistor_SMD:R_0603_1608Metric
- R30, R31: footprint Resistors_SMD:R_0603 -> Resistor_SMD:R_0603_1608Metric; moved to B.Cu
- R4: value 4k7 -> 2K; footprint Resistors_SMD:R_0603 -> Resistor_SMD:R_0603_1608Metric
- U1: footprint Housings_SSOP:TSSOP-16-1EP_4.4x5mm_Pitch0.65mm -> Package_SO:TSSOP-16-1EP_4.4x5mm_P0.65mm
- U2: value LTV-847 -> PC817; footprint Housings_DIP:DIP-16_W8.89mm_SMDSocket_LongPads -> Package_SO:SOP-4_4.4x2.8mm_P1.27mm
- U3: value LTV-847 -> NRF24L01_Breakout; footprint Housings_DIP:DIP-16_W8.89mm_SMDSocket_LongPads -> Connector_PinHeader_2.54mm:PinHeader_2x04_P2.54mm_Vertical
- U4: value LTV-847 -> Bluetooth_HC-05; footprint Housings_DIP:DIP-16_W8.89mm_SMDSocket_LongPads -> Bluetooth:Bluetooth_HC-05
- U5: footprint Housings_SOIC:SOIC-20W_7.5x12.8mm_Pitch1.27mm -> Package_SO:SOIC-20W_7.5x12.8mm_P1.27mm
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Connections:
- C1 pad 1: Net-(C1-Pad1) -> +5V
- C2 pad 1: Net-(C2-Pad1) -> +5V
- C5 pad 1: +5V -> GND
- C5 pad 2: GND -> Net-(C5-Pad2)
- C6 pad 1: +5V -> GND
- C6 pad 2: GND -> Net-(C6-Pad2)
- C8 pad 1: +12V -> AX_PWR
- D1 pad 1: GND -> Net-(D1-Pad1)
- D1 pad 2: Net-(D1-Pad2) -> GND
- D2 pad 1: GND -> Net-(D2-Pad1)
- D2 pad 2: Net-(D2-Pad2) -> GND
- J1 pad 1: +12V -> Net-(J1-Pad1)
- J1 pad 2: GND -> Net-(J1-Pad2)
- J1 pad 3: SENS1 -> Net-(J1-Pad3)
- J10 pad 1: +12V -> +5V
- J10 pad 2: R4 -> JUMPER
- J10 pad 3: +5VA -> SIDE
- J11 pad 1: +12V -> GND
- J11 pad 2: R5 -> Net-(J11-Pad2)
- J11 pad 3: +5VA -> +12V
- J12 pad 1: +12V -> +5V
- J12 pad 2: R6 -> TACTIC2
- J12 pad 3: +5VA -> TACTIC1
- J13 pad 1: +12V -> +5V
- J13 pad 2: GND -> SCL
- J13 pad 3: SW1 -> SDA
- J14 pad 1: +12V -> GND
- J14 pad 2: GND -> SER_RX
- J14 pad 3: SW2 -> SER_TX
- J15 pad 1: +12V -> Net-(J15-Pad1)
- J15 pad 2: GND -> Net-(J15-Pad2)
- J15 pad 3: SW3 -> GND
- J17 pad 1: +12V -> GND
- J17 pad 2: GND -> Net-(J17-Pad2)
- J17 pad 3: SW5 -> +12V
- J18 pad 1: +12V -> GND
- J18 pad 2: GND -> Net-(J18-Pad2)
- J18 pad 3: SW6 -> +12V
- J19 pad 2: GND -> PWM1
- J19 pad 3: PWM1 -> GND
- J2 pad 1: +12V -> AX_PWR
- J2 pad 2: GND -> AX_PWR
- J2 pad 3: SENS2 -> AX_SIGNAL
- J20 pad 2: GND -> PWM2
- J20 pad 3: PWM2 -> GND
- J21 pad 1: +5VA -> +12V
- J21 pad 2: GND -> _S2
- J22 pad 1: GND -> +12V
- J22 pad 2: SCL -> _S3
- J23 pad 1: GND -> Net-(D4-Pad2)
- J23 pad 2: Net-(J23-Pad2) -> GND
- J24 pad 1: GND -> Net-(J24-Pad1)
- J24 pad 2: Net-(J24-Pad2) -> GND
- J25 pad 1: GND -> Net-(J25-Pad1)
- J25 pad 2: Net-(D4-Pad2) -> GND
- J26 pad 1: GND -> +12V
- J26 pad 2: CANL -> _S4
- J27 pad 1: GND -> +12V
- J27 pad 2: CANL -> _S5
- J28 pad 1: +5V -> +12V
- J28 pad 2: +5V -> _S6
- J3 pad 1: +12V -> +5V
- J3 pad 2: GND -> BIN_SEN1
- J3 pad 3: SENS3 -> GND
- J30 pad 1: +12V -> GND
- J30 pad 2: AX_SIGNAL -> Net-(J30-Pad2)
- J30 pad 3: GND -> +12V
- J31 pad 2: GND -> Net-(J31-Pad2)
- J31 pad 3: GND -> +12V
- J32 pad 1: Net-(J32-Pad1) -> GND
- J32 pad 3: Net-(J32-Pad3) -> +12V
- J33 pad 1: Net-(J33-Pad1) -> +5VA
- J33 pad 2: Net-(J33-Pad2) -> PWM3
- J33 pad 3: Net-(J33-Pad3) -> GND
- J4 pad 1: +12V -> +5V
- J4 pad 2: GND -> BIN_SEN4
- J4 pad 3: SENS4 -> GND
- J5 pad 2: GND -> _S1
- J6 pad 1: +12V -> +5V
- J6 pad 2: GND -> BIN_SEN2
- J6 pad 3: SENS6 -> GND
- J7 pad 1: +12V -> +5V
- J7 pad 2: R1 -> BIN_SEN5
- J7 pad 3: +5VA -> GND
- J8 pad 1: +12V -> +5V
- J8 pad 2: R2 -> BIN_SEN3
- J8 pad 3: +5VA -> GND
- J9 pad 1: +12V -> +5V
- J9 pad 2: R3 -> BIN_SEN6
- J9 pad 3: +5VA -> GND
- K1 pad 2: (no net) -> Net-(D1-Pad1)
- K1 pad 3: (no net) -> +12V
- K1 pad 5: R1 -> +12V
- K2 pad 2: (no net) -> Net-(D2-Pad1)
- K2 pad 3: (no net) -> +12V
- K2 pad 5: R2 -> +12V
- Q1 pad 3: Net-(J23-Pad2) -> Net-(J24-Pad1)
- Q2 pad 3: Net-(J24-Pad2) -> Net-(J25-Pad1)
- R1 pad 1: GND -> +12V
- R1 pad 2: Net-(R1-Pad2) -> Net-(J11-Pad2)
- R10 pad 1: SWO_2 -> SENSOR1
- R11 pad 1: GND -> Net-(J17-Pad2)
- R12 pad 1: SWO_1 -> Net-(J18-Pad2)
- R12 pad 2: GND -> Net-(R12-Pad2)
- R13 pad 1: GND -> Net-(J11-Pad2)
- R14 pad 1: SO_6 -> SENSOR3
- R15 pad 1: GND -> SENSOR5
- R15 pad 2: Net-(R15-Pad2) -> GND
- R16 pad 1: SO_5 -> +12V
- R16 pad 2: GND -> Net-(J30-Pad2)
- R17 pad 2: Net-(R17-Pad2) -> Net-(J30-Pad2)
- R18 pad 1: SWO_6 -> +12V
- R18 pad 2: GND -> Net-(J31-Pad2)
- R19 pad 2: Net-(R19-Pad2) -> Net-(J31-Pad2)
- R2 pad 1: SO_4 -> GND
- R2 pad 2: GND -> Net-(J11-Pad2)
- R20 pad 1: SWO_5 -> +12V
- R20 pad 2: GND -> Net-(J32-Pad2)
- R21 pad 2: Net-(R21-Pad2) -> Net-(J32-Pad2)
- R22 pad 1: SWO_4 -> Net-(J30-Pad2)
- R22 pad 2: GND -> Net-(R22-Pad2)
- R23 pad 1: GND -> Net-(J31-Pad2)
- R24 pad 1: SWO_3 -> Net-(J32-Pad2)
- R24 pad 2: GND -> Net-(R24-Pad2)
- R25 pad 1: +5V -> SENSOR2
- R25 pad 2: Net-(D1-Pad2) -> GND
- R26 pad 1: +5VA -> SENSOR4
- R26 pad 2: Net-(D2-Pad2) -> GND
- R27 pad 1: +12V -> SENSOR6
- R27 pad 2: Net-(D3-Pad2) -> GND
- R28 pad 1: Net-(IC1-Pad9) -> Net-(D3-Pad2)
- R28 pad 2: +5V -> +12V
- R29 pad 1: CANH -> Net-(D5-Pad2)
- R29 pad 2: CANL -> +5V
- R3 pad 1: GND -> DBG_TX
- R4 pad 1: SO_3 -> Net-(R3-Pad2)
- R5 pad 1: GND -> +5V
- R6 pad 1: SO_2 -> +12V
- R6 pad 2: GND -> Net-(J17-Pad2)
- R7 pad 2: Net-(R7-Pad2) -> Net-(J17-Pad2)
- R8 pad 1: SO_1 -> +12V
- R8 pad 2: GND -> Net-(J18-Pad2)
- R9 pad 2: Net-(R9-Pad2) -> Net-(J18-Pad2)
- U1 pad 10: (no net) -> Net-(U1-Pad10)
- U1 pad 11: R6_SIG -> Net-(U1-Pad11)
- U1 pad 12: R5_SIG -> Net-(U1-Pad12)
- U1 pad 13: R4_SIG -> R2_SIG
- U1 pad 14: R3_SIG -> R2_SIG
- U1 pad 15: R2_SIG -> R1_SIG
- U1 pad 2: R2_CONT -> R1_CONT
- U1 pad 3: R3_CONT -> R2_CONT
- U1 pad 4: R4_CONT -> R2_CONT
- U1 pad 5: R5_CONT -> Net-(U1-Pad5)
- U1 pad 6: R6_CONT -> Net-(U1-Pad6)
- U1 pad 7: (no net) -> Net-(U1-Pad7)
- U1 pad 9: +5VA -> +12V
- U2 pad 1: SENS1 -> Net-(R13-Pad2)
- U2 pad 2: Net-(R7-Pad2) -> GND
- U2 pad 3: SENS2 -> SENSOR1
- U2 pad 4: Net-(R5-Pad2) -> +5V
- U3 pad 1: SENS5 -> GND
- U3 pad 2: Net-(R15-Pad2) -> +3V3
- U3 pad 3: SENS6 -> NRF_CE
- U3 pad 4: Net-(R13-Pad2) -> NRF_CS
- U3 pad 5: SW1 -> CAN_SCK
- U3 pad 6: Net-(R11-Pad2) -> CAN_MOSI
- U3 pad 7: SW2 -> CAN_MISO
- U3 pad 8: Net-(R9-Pad2) -> Net-(U3-Pad8)
- U4 pad 2: Net-(R23-Pad2) -> Net-(R3-Pad2)
- U4 pad 3: SW4 -> DBG_RX
- U4 pad 4: Net-(R21-Pad2) -> GND
- U4 pad 5: SW5 -> +5V
- U5 pad 11: (no net) -> Net-(U5-Pad11)
- U5 pad 12: (no net) -> Net-(U5-Pad12)
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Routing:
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- added copper zone on F.Cu, net +5VA
- added copper zone on F.Cu, net Net-(D1-Pad1)
- added copper zone on F.Cu, net Net-(D2-Pad1)
- added copper zone on F.Cu, net Net-(J24-Pad1)
- added copper zone on F.Cu, net Net-(J25-Pad1)
- removed copper zone on F.Cu, net +5V
- removed copper zone on F.Cu, net Net-(J23-Pad2)
- removed copper zone on F.Cu, net Net-(J24-Pad2)
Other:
- board size 131.6 x 66.5 mm -> 88.6 x 64.4 mm
- board text added: "+ -"
- board text added: "1"
- board text added: "12V SIG GND"
- board text added: "2"
- board text added: "3"
- board text added: "4"
- board text added: "5"
- board text added: "6"
- board text added: "A15"
- board text added: "A6"
- board text added: "AX-12"
- board text added: "BINARY 1 GND SIG +5V"
- board text added: "BINARY 2 GND SIG +5V"
- board text added: "BINARY 3 GND SIG +5V"
- board text added: "BINARY 4 GND SIG +5V"
- board text added: "BINARY 5 GND SIG +5V"
- board text added: "BINARY 6 GND SIG +5V"
- board text added: "CAN Bus"
- board text added: "CNH CNL GND"
- board text added: "Developed by Silard Gal at"
- board text added: "GND SDA SCL +5V"
- board text added: "GND SDE JUM +5V"
- board text added: "GND SIG +5V"
- board text added: "GND SIG PWR PWR"
- board text added: "GND TC1 TC2 +5V"
- board text added: "Mainboard V1 | 2018 Dec"
- board text added: "Mainboard V1.0 - Dec 2018"
- board text added: "NRF24L01"
- board text added: "RX"
- board text added: "Relay 1"
- board text added: "Relay 2"
- board text added: "SIG 12V"
- board text added: "STX SRX GND"
- board text added: "VCC"
- board text removed: "#1"
- board text removed: "#2"
- board text removed: "#3"
- board text removed: "AX-12 SECTION"
- board text removed: "CAN SECTION"
- board text removed: "CANH"
- board text removed: "CANL"
- board text removed: "D22"
- board text removed: "D23"
- board text removed: "D24"
- board text removed: "D25"
- board text removed: "D26"
- board text removed: "D27"
- board text removed: "D28"
- board text removed: "D29"
- board text removed: "D30"
- board text removed: "D32"
- board text removed: "D33"
- board text removed: "D34"
- board text removed: "D35"
- board text removed: "D36"
- board text removed: "D37"
- board text removed: "D38"
- board text removed: "D39"
- board text removed: "D40"
- board text removed: "Designed by Silard Gal"
- board text removed: "EXTRA PINS SECTION"
- board text removed: "GND"
- board text removed: "I2C SECTION"
- board text removed: "Mainboard SEPTEMBER 2018"
- board text removed: "S"
- board text removed: "S1"
- board text removed: "S2"
- board text removed: "S3"
- board text removed: "S4"
- board text removed: "S5"
- board text removed: "S6"
- board text removed: "SCL"
- board text removed: "SDA"
- board text removed: "SERVO SECTION"
- board text removed: "SIG"
- board text removed: "SIGNAL POWER SECTION"
- board text removed: "VCC 5V"
- board text removed: "W1"
- board text removed: "W2"
- board text removed: "W3"
- board text removed: "W4"
- board text removed: "W5"
- board text removed: "W6"

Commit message: Readme and images
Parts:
- removed the XA1 at (92.8, 127.9) (x2)
- added XA1 (x2): Arduino_Mega2560_Shield, Arduino:Arduino_Mega2560_Shield, F.Cu at (92.8, 127.9)
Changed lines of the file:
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@@
-(kicad_pcb (version 20171130) (host pcbnew 5.0.1-33cea8e~68~ubuntu18.04.1)
+(kicad_pcb (version 20171130) (host pcbnew "(6.0.0-rc1-dev-1469-gd619da17c)")
   (general
     (thickness 1.6)
@@
   )
   (setup
-    (last_trace_width 1)
+    (last_trace_width 0.25)
     (user_trace_width 0.4)
     (user_trace_width 0.5)
@@
     (zone_45_only yes)
     (trace_min 0.2)
-    (segment_width 0.2)
-    (edge_width 0.15)
     (via_size 0.6)
     (via_drill 0.4)
@@
     (uvia_min_size 0.2)
     (uvia_min_drill 0.1)
+    (edge_width 0.15)
+    (segment_width 0.2)
     (pcb_text_width 0.3)
     (pcb_text_size 1.5 1.5)
@@
     (pad A0 smd rect (at 50.8 -0.762 90) (size 2.51 1) (layers B.Cu B.Paste B.Mask)
       (net 9 BIN_SEN1))
-    (model Pin_Headers.3dshapes/Pin_Header_Straight_1x10_Pitch2.54mm_SMD_Pin1Right.wrl
-      (offset (xyz 30.22599954605102 50.79999923706055 -1.523999977111816))
-      (scale (xyz 1 1 1))
-      (rotate (xyz 180 0 90))
-    )
-    (model Pin_Headers.3dshapes/Pin_Header_Straight_1x08_Pitch2.54mm_SMD_Pin1Right.wrl
-      (offset (xyz 54.60999917984009 50.79999923706055 -1.523999977111816))
-      (scale (xyz 1 1 1))
-      (rotate (xyz 180 0 90))
-    )
-    (model Pin_Headers.3dshapes/Pin_Header_Straight_1x08_Pitch2.54mm_SMD_Pin1Right.wrl
-      (offset (xyz 77.46999883651733 50.79999923706055 -1.523999977111816))
-      (scale (xyz 1 1 1))
-      (rotate (xyz 180 0 90))
-    )
-    (model Pin_Headers.3dshapes/Pin_Header_Straight_1x08_Pitch2.54mm_SMD_Pin1Right.wrl
-      (offset (xyz 36.8299994468689 2.539999961853027 -1.523999977111816))
-      (scale (xyz 1 1 1))
-      (rotate (xyz 180 0 90))
-    )
-    (model Pin_Headers.3dshapes/Pin_Header_Straight_1x08_Pitch2.54mm_SMD_Pin1Right.wrl
-      (offset (xyz 59.68999910354614 2.539999961853027 -1.523999977111816))
-      (scale (xyz 1 1 1))
-      (rotate (xyz 180 0 90))
-    )
-    (model Pin_Headers.3dshapes/Pin_Header_Straight_1x08_Pitch2.54mm_SMD_Pin1Right.wrl
-      (offset (xyz 82.54999876022339 2.539999961853027 -1.523999977111816))
-      (scale (xyz 1 1 1))
-      (rotate (xyz 180 0 90))
-    )
-    (model Pin_Headers.3dshapes/Pin_Header_Straight_2x18_Pitch2.54mm_SMD.wrl
-      (offset (xyz 95.24999856948853 29.20999956130981 -1.523999977111816))
-      (scale (xyz 1 1 1))
-      (rotate (xyz 180 0 180))
-    )
   )
   (module Capacitor_SMD:C_0603_1608Metric (layer F.Cu)
